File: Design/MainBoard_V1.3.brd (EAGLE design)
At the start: 120.7 x 81.2 mm, 92 parts, among them P4SMA-4 TVS, P4SMA_1 TVS, P4SMA_2 TVS, P4SMA_3 TVS, P4SMA_4 TVS, P4SMA_5 TVS, P4SMA_6 TVS, T1 NDS352AP, U1 STM32F20XR, U2 MicroSDCard

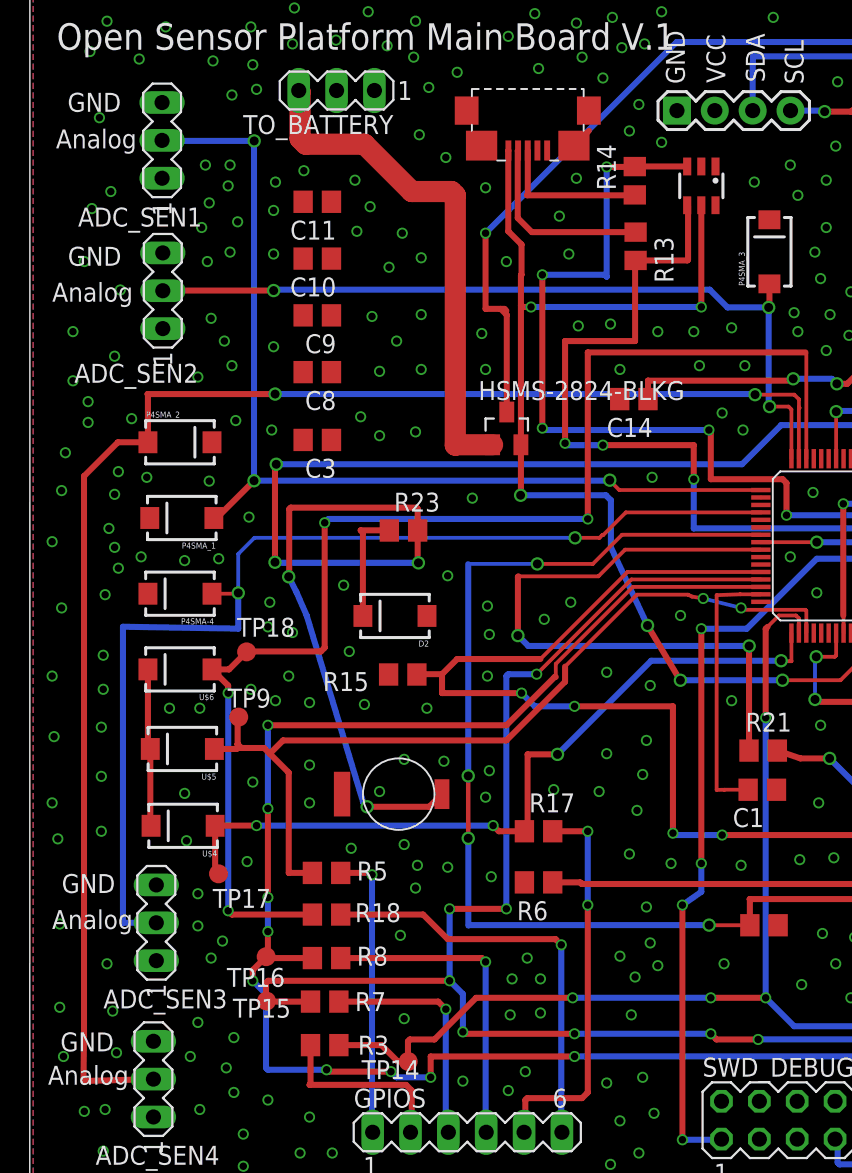
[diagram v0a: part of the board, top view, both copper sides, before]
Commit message: Updated schematics and boards
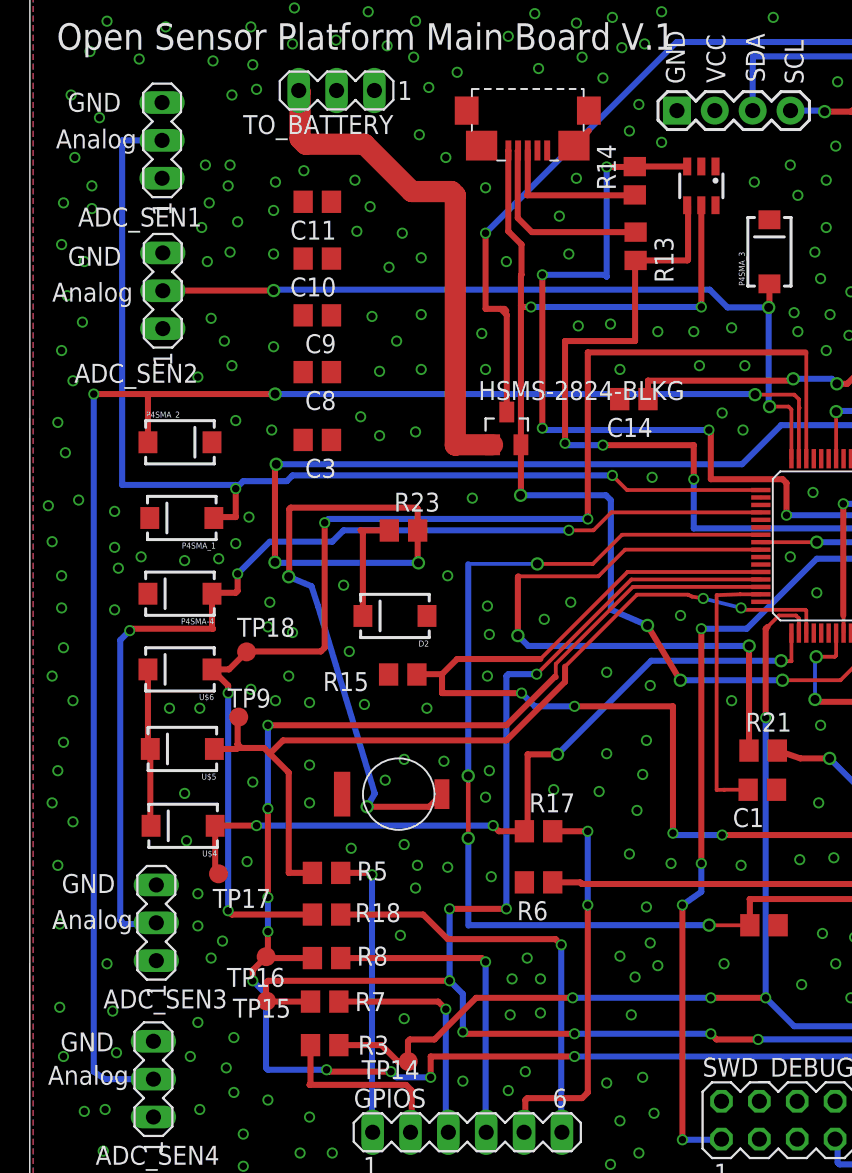
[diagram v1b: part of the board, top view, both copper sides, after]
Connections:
- net ADC1_IN1: now also ADC_SEN1.2, P4SMA_1.A, U1.17; no longer ADC_SEN4.2, P4SMA_2.A, U1.15
- net ADC1_IN3: now also ADC_SEN3.2, P4SMA-4.A, U1.20; no longer ADC_SEN1.2, P4SMA_1.A, U1.17
- net ADC1_IN4: now also ADC_SEN4.2, P4SMA_2.A, U1.15; no longer ADC_SEN3.2, P4SMA-4.A, U1.20
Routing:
- net ADC1_IN4: track 72.9 -> 104.4 mm, vias 2 -> 3
- net ADC1_IN1: track 101.6 -> 73.1 mm
- net ADC1_IN3: track 67.1 -> 70.0 mm
- net VBUS/FS: track 183.8 -> 184.8 mm
- net VBAT: track 100.1 -> 101.0 mm
